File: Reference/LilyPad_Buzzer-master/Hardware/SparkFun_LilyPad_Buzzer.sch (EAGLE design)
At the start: 8 parts

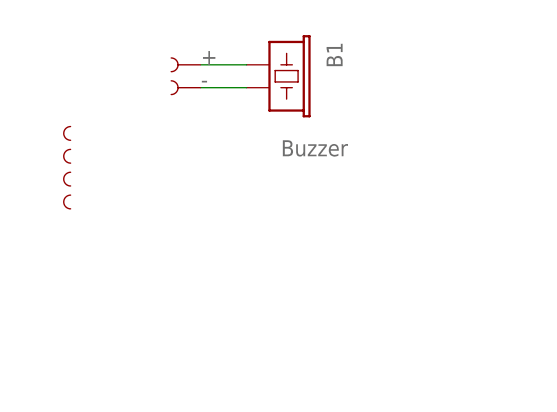
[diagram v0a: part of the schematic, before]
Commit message: v35 ready for initial review
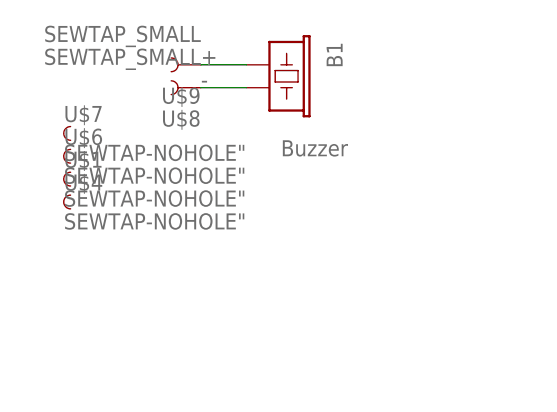
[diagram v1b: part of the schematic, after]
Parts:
- U$1, U$4, U$6, U$7: value SEWTAP-NOHOLE2 -> SEWTAP-NOHOLE"; device LilyPad-Wearables:SEWTAP-NOHOLE2 -> LilyPad-Wearables:SEWTAP-NOHOLE"
- U$8, U$9: value SEWTAP6 -> SEWTAP_SMALL; device LilyPad-Wearables:SEWTAP6 -> LilyPad-Wearables:SEWTAP_SMALL
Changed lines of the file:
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@@
 <?xml version="1.0" encoding="utf-8"?>
 <!DOCTYPE eagle SYSTEM "eagle.dtd">
-<eagle version="7.2.0">
+<eagle version="7.7.0">
 <drawing>
 <settings>
@@
 <layer number="121" name="_tsilk" color="7" fill="1" visible="yes" active="yes"/>
 <layer number="122" name="_bsilk" color="7" fill="1" visible="yes" active="yes"/>
+<layer number="125" name="_tNames" color="7" fill="1" visible="yes" active="yes"/>
 <layer number="144" name="Drill_legend" color="7" fill="1" visible="yes" active="yes"/>
 <layer number="151" name="HeatSink" color="7" fill="1" visible="yes" active="yes"/>
@@
 <parts>
 <part name="FRAME1" library="SparkFun" deviceset="FRAME-LETTER" device=""/>
-<part name="U$1" library="LilyPad-Wearables" deviceset="SEWTAP-NOHOLE" device="2"/>
-<part name="U$6" library="LilyPad-Wearables" deviceset="SEWTAP-NOHOLE" device="2"/>
-<part name="U$7" library="LilyPad-Wearables" deviceset="SEWTAP-NOHOLE" device="2"/>
-<part name="U$8" library="LilyPad-Wearables" deviceset="SEWTAP" device="6"/>
-<part name="U$9" library="LilyPad-Wearables" deviceset="SEWTAP" device="6"/>
-<part name="U$4" library="LilyPad-Wearables" deviceset="SEWTAP-NOHOLE" device="2"/>
+<part name="U$1" library="LilyPad-Wearables" deviceset="SEWTAP-NOHOLE" device="&quot;"/>
+<part name="U$6" library="LilyPad-Wearables" deviceset="SEWTAP-NOHOLE" device="&quot;"/>
+<part name="U$7" library="LilyPad-Wearables" deviceset="SEWTAP-NOHOLE" device="&quot;"/>
+<part name="U$8" library="LilyPad-Wearables" deviceset="SEWTAP" device="_SMALL" value="SEWTAP_SMALL"/>
+<part name="U$9" library="LilyPad-Wearables" deviceset="SEWTAP" device="_SMALL" value="SEWTAP_SMALL"/>
+<part name="U$4" library="LilyPad-Wearables" deviceset="SEWTAP-NOHOLE" device="&quot;"/>
 <part name="U$2" library="LilyPad-Wearables" deviceset="LOGO-LP" device="LP"/>
 <part name="B1" library="SparkFun" deviceset="BUZZER" device="SMD2" value="Buzzer"/>
